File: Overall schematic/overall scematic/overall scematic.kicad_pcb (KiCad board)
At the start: 2 copper layers, 100 x 100 mm, 45 parts, among them IC1 battery protection IC DW01A-G, J1 USB_B_Micro, J12 Conn_01x24_Socket, J13 Conn_01x24_Socket, J19 Conn_01x02_Pin, J2 Conn_01x02_Pin, J3 Battery Charger IC TP4056, J4 Conn_01x02_Pin, J5 Conn_01x02_Pin, J6 Conn_01x02_Pin, J7 Conn_01x02_Pin, J9 Conn_02x24_Counter_Clockwise, Q1 Dual Mosfet FS8205A, SW1 SW_Push, U1 MCP1700T-3302E_TT, U2 HDC1080, U3 STLINK_UCT, U4 AT24CS01-STUM, U5 MCP9701AT-E_TT

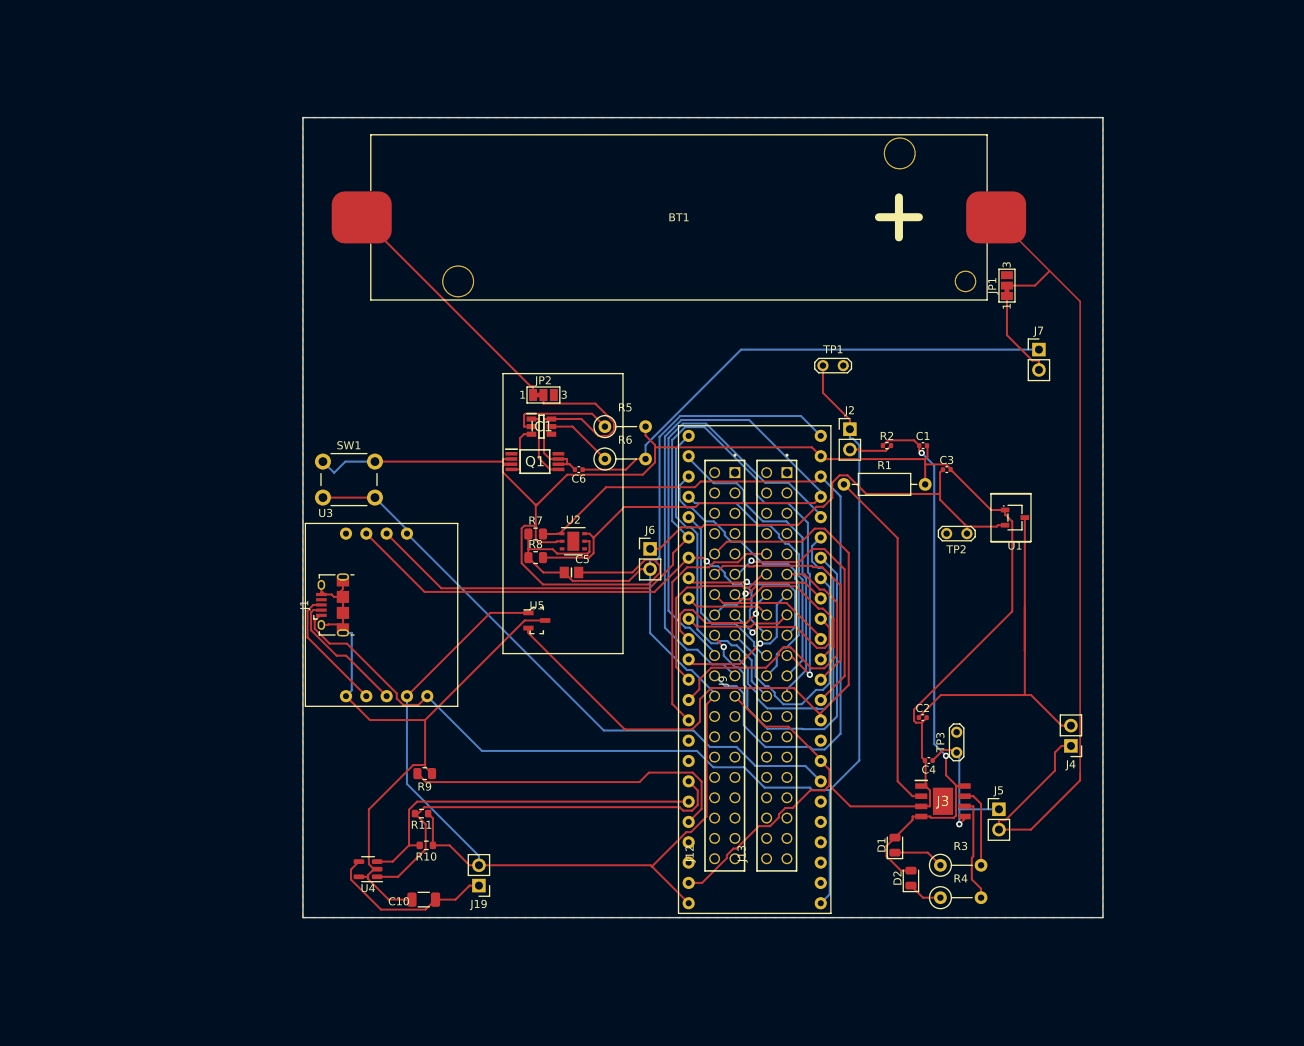
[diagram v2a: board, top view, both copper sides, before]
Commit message: hello
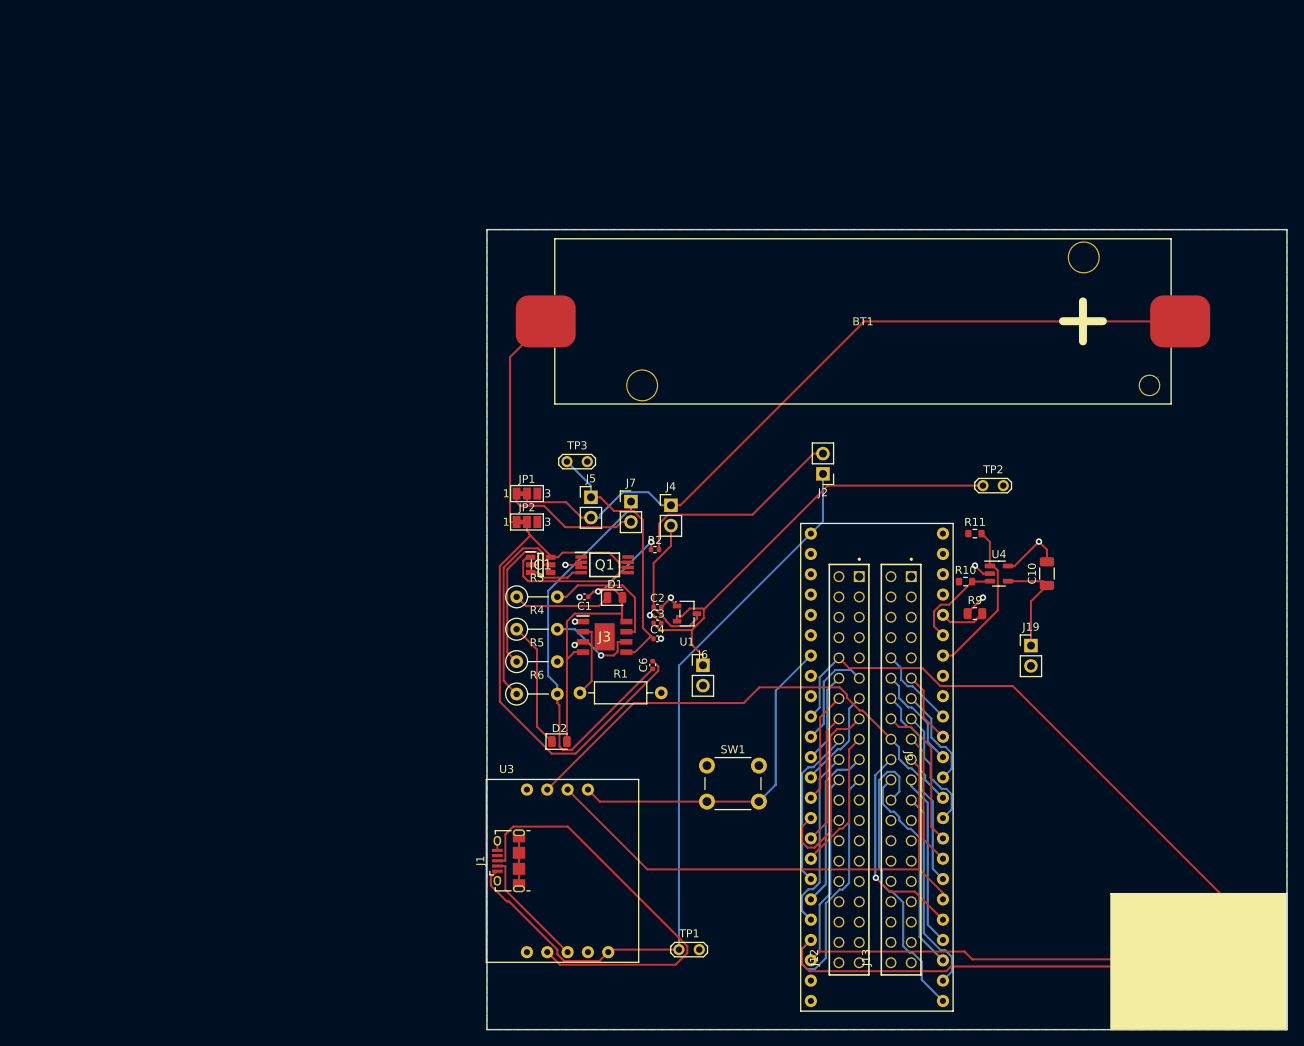
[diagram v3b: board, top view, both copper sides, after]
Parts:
- moved U5 101.3 mm to (205.9, 148.0)
- moved U2 93.0 mm to (198.6, 142.1)
- moved C5 92.6 mm to (197.1, 147.0)
- moved R7 92.6 mm to (192.6, 142.2)
- moved R8 92.6 mm to (192.6, 145.1)
- moved C10 87.9 mm to (180.0, 95.0), turned to 90 degrees
- moved U4 87.1 mm to (174.0, 95.0), turned to 0 degrees
- moved R11 77.5 mm to (171.0, 90.0), turned to 0 degrees
- moved J19 75.2 mm to (178.0, 104.0), turned to 0 degrees
- moved TP1 75.2 mm to (134.0, 142.0)
- moved R10 75.0 mm to (169.8, 96.0), turned to 0 degrees
- moved R9 71.6 mm to (171.0, 100.0), turned to 0 degrees
- moved JP1 65.4 mm to (115.0, 85.0), turned to 0 degrees
- moved J5 64.2 mm to (123.0, 85.5)
- moved R3 62.7 mm to (113.7, 97.9)
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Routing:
- net GND: track 339.8 -> 30.6 mm, vias 0 -> 13
- net /Supply_Voltage: track 197.6 -> 1.94 mm, vias 0 -> 1
- net Vreg_Out: track 147.4 -> 97.4 mm
- net /Micro controller pin outs/BOOT: track 43.8 -> 6.11 mm
- net Data +: track 15.8 -> 53.2 mm
- net /Micro controller pin outs/PA9: track 103.8 -> 67.2 mm, vias 1 -> 0
- net Net-(IC1-GND): track 32.2 -> 68.4 mm
- net Net-(J3-PROG2): track 43.6 -> 9.33 mm
- net /Micro controller pin outs/NRST: track 77.2 -> 42.9 mm
- net /Micro controller pin outs/PB7: track 46.0 -> 12.0 mm
- net /Micro controller pin outs/PB6: track 52.0 -> 19.9 mm
- net /Micro controller pin outs/PB2: track 54.7 -> 22.8 mm
- net Net-(J4-Pin_2): track 49.5 -> 18.7 mm
- net /Micro controller pin outs/PA15: track 38.3 -> 8.96 mm
- net /Power module/Vcc_IC: track 70.0 -> 43.5 mm
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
